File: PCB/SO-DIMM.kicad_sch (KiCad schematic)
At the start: 1 part, among them J1 SODIMM-260_Split

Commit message: Fix broken CM4IO/SODIMM library links and add missing footprints
Both fp-lib-table and sym-lib-table pointed to other collaborators'
absolute local paths (a Windows user path and a Linux path), so the
CM4IO and SODIMM libraries could not resolve on this machine at all.
Repointed both tables at the project's own libraries/ folder using
${KIPRJMOD}-relative paths.

- Added the missing SODIMM_DDR4_EDGE footprint (260-pin card edge)
  and split the combined CM4 mezzanine footprint into
  Raspberry-Pi-4-Compute-Module-A/-B to match the schematic's
  existing per-connector pin numbering (1-100 / 101-200)
- Added Connectors.pretty and MCP25625T_E_ML.pretty footprint
  libraries that were referenced but never committed
- Moved the Mezzanine_A/Mezzanine_B symbols out of the orphaned
  "kai-library" reference (which pointed to no actual file) into
  the existing CM4IO symbol library
- Corrected Module1/Module2 MPN/Digi-Key part numbers to the
  primary DF40HC(3.0)-100DS-0.4V variant, keeping the old
  DF40C-100DS-0.4V values as (Alt) fields
- Reverted an in-progress SO-DIMM.kicad_sch rework that had
  misrouted 8 PCIe signals to the wrong physical pins and silently
  disconnected the CSI/USB3 nets, restoring the known-good pinout
  while keeping the CM4IO footprint rename

Co-Authored-By: Claude Sonnet 5 <noreply@anthropic.com>
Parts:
- J1: footprint kai's library:SODIMM_DDR4_EDGE -> CM4IO:SODIMM_DDR4_EDGE
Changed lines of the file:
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@@
 			)
 		)
-		(property "Footprint" "kai's library:SODIMM_DDR4_EDGE"
+		(property "Footprint" "CM4IO:SODIMM_DDR4_EDGE"
 			(at 396.24 156.21 0)
 			(hide yes)
@@
 			)
 		)
-		(property "Footprint" "kai's library:SODIMM_DDR4_EDGE"
+		(property "Footprint" "CM4IO:SODIMM_DDR4_EDGE"
 			(at 147.32 148.59 0)
 			(hide yes)
@@
 			)
 		)
-		(property "Footprint" "kai's library:SODIMM_DDR4_EDGE"
+		(property "Footprint" "CM4IO:SODIMM_DDR4_EDGE"
 			(at 229.87 71.12 0)
 			(hide yes)
@@
 			)
 		)
-		(property "Footprint" "kai's library:SODIMM_DDR4_EDGE"
+		(property "Footprint" "CM4IO:SODIMM_DDR4_EDGE"
 			(at 312.42 71.12 0)
 			(hide yes)
@@
 			)
 		)
-		(property "Footprint" "kai's library:SODIMM_DDR4_EDGE"
+		(property "Footprint" "CM4IO:SODIMM_DDR4_EDGE"
 			(at 130.81 62.23 0)
 			(hide yes)
@@
 			)
 		)
-		(property "Footprint" "kai's library:SODIMM_DDR4_EDGE"
+		(property "Footprint" "CM4IO:SODIMM_DDR4_EDGE"
 			(at 394.97 71.12 0)
 			(hide yes)
@@
 			)
 		)
-		(property "Footprint" "kai's library:SODIMM_DDR4_EDGE"
+		(property "Footprint" "CM4IO:SODIMM_DDR4_EDGE"
 			(at 276.86 156.21 0)
 			(hide yes)

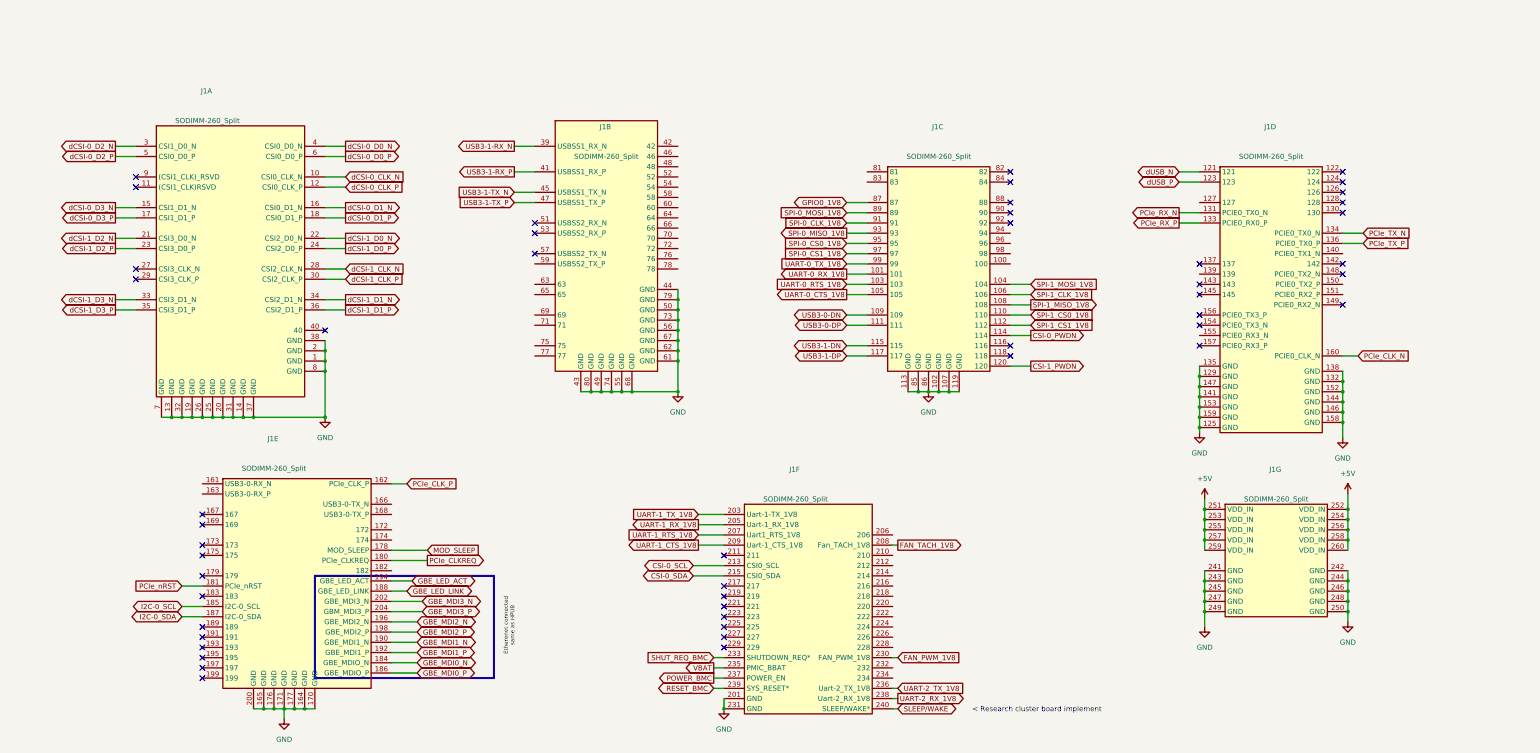
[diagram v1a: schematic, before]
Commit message: Add CAN/PCIe wake signals, drop USB3/CSI-1/most of SPI-1, route GbE pairs
Schematic changes (confirmed intentional):
- Renamed dCSI-0_D2/D3_N/P to CSI-0_D2/D3_N/P (same pins, label cleanup)
- Added CAN_RX/CAN_TX on J1 pins 143/145
- Added PCIe_WAKE_N on J1 pin 179 / Module1 pin 104 (repurposed from
  SPI-1_MOSI_1V8)
- Removed USB3-0 and USB3-1 (both ports entirely), the second CSI
  camera interface (dCSI-1, 10 signals), the remaining 4 SPI-1
  signals, and CSI-0/CSI-1_PWDN

PCB changes:
- Added carrier.kicad_dru with GbE differential pair rules: intra-pair
  skew <=0.25mm (1000BASE-T MDI tolerance) and inter-pair length
  matched to 49.7-50.7mm, both validated against kicad-cli pcb drc
- In-progress length tuning on the 4 GBE_MDI differential pairs

Co-Authored-By: Claude Sonnet 5 <noreply@anthropic.com>
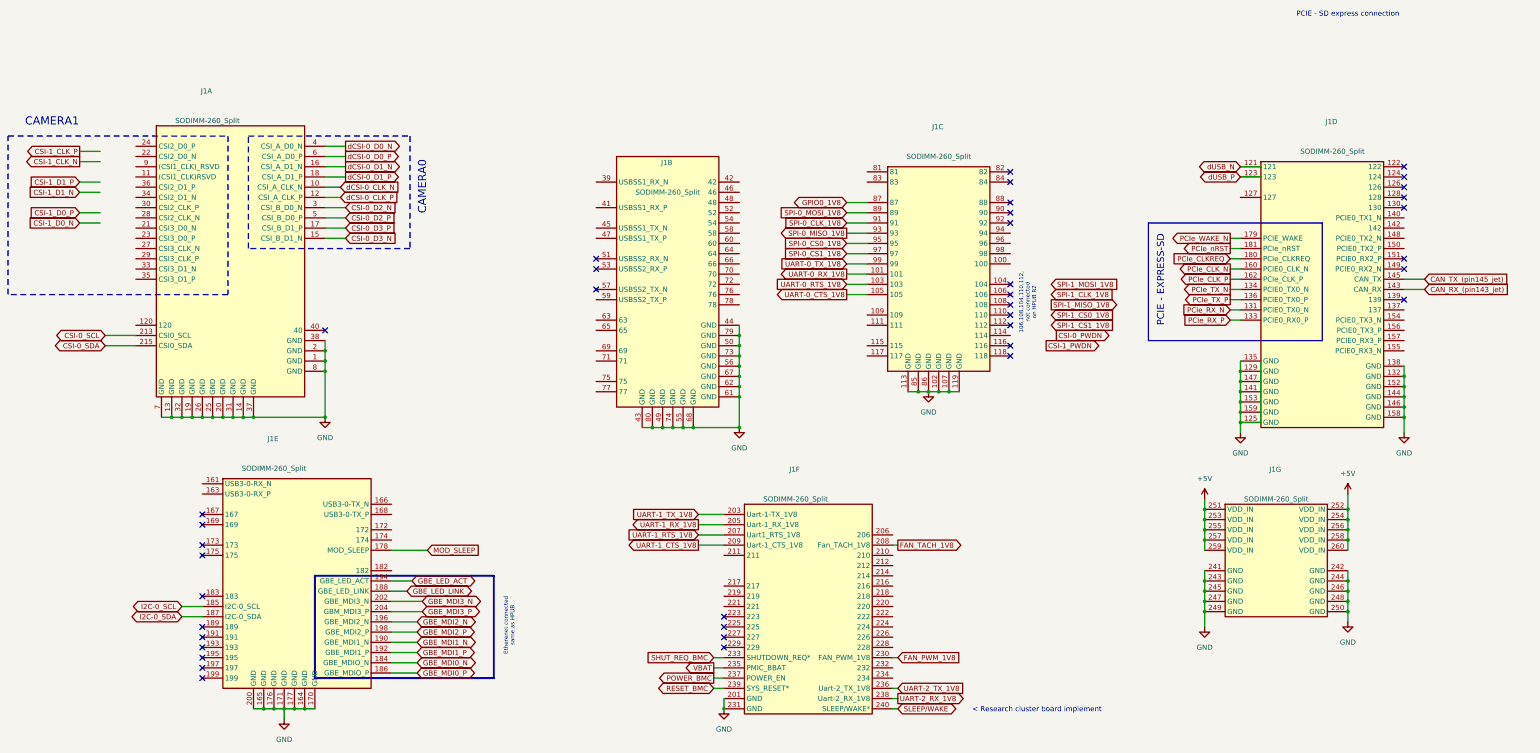
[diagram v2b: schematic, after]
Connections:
- net CSI-0_PWDN: no longer J1.114
- net CSI-0_SCL: now also J1.213 (CSI0_SCL); no longer J1.213 (CSI0_SCL)
- net CSI-0_SDA: now also J1.215 (CSI0_SDA); no longer J1.215 (CSI0_SDA)
- net CSI-1_PWDN: no longer J1.120
- net PCIe_CLKREQ: now also J1.180 (PCIe_CLKREQ); no longer J1.180 (PCIe_CLKREQ)
- net PCIe_CLK_P: now also J1.162 (PCIe_CLK_P); no longer J1.162 (PCIe_CLK_P)
- net PCIe_nRST: now also J1.181 (PCIe_nRST); no longer J1.181 (PCIe_nRST)
- net SPI-1_CLK_1V8: no longer J1.106
- net SPI-1_CS0_1V8: no longer J1.110
- net SPI-1_CS1_1V8: no longer J1.112
- net SPI-1_MISO_1V8: no longer J1.108
- net SPI-1_MOSI_1V8: no longer J1.104
- net CAN_RX_(pin143_jet): now reaches J1.143 (CAN_RX)
- net CAN_TX_(pin145_jet): now reaches J1.145 (CAN_TX)
- net USB3-0-DN: no longer names the net of J1.109
- net USB3-0-DP: no longer names the net of J1.111
- net USB3-1-DN: no longer names the net of J1.115
- net USB3-1-DP: no longer names the net of J1.117
- net USB3-1-RX_N: no longer names the net of J1.39 (USBSS1_RX_N)
- net USB3-1-RX_P: no longer names the net of J1.41 (USBSS1_RX_P)
- net USB3-1-TX_N: no longer names the net of J1.45 (USBSS1_TX_N)
- net USB3-1-TX_P: no longer names the net of J1.47 (USBSS1_TX_P)
- net dCSI-0_D2_N renamed CSI-0_D2_N
- net dCSI-0_D2_P renamed CSI-0_D2_P
- net dCSI-0_D3_N renamed CSI-0_D3_N
- net dCSI-0_D3_P renamed CSI-0_D3_P
- net dCSI-1_CLK_N: no longer names the net of J1.28 (CSI2_CLK_N)
- net dCSI-1_CLK_P: no longer names the net of J1.30 (CSI2_CLK_P)
- net dCSI-1_D0_N: no longer names the net of J1.22 (CSI2_D0_N)
- net dCSI-1_D0_P: no longer names the net of J1.24 (CSI2_D0_P)
- net dCSI-1_D1_N: no longer names the net of J1.34 (CSI2_D1_N)
- net dCSI-1_D1_P: no longer names the net of J1.36 (CSI2_D1_P)
- net dCSI-1_D2_N: no longer names the net of J1.21 (CSI3_D0_N)
- net dCSI-1_D2_P: no longer names the net of J1.23 (CSI3_D0_P)
- net dCSI-1_D3_N: no longer names the net of J1.33 (CSI3_D1_N)
- net dCSI-1_D3_P: no longer names the net of J1.35 (CSI3_D1_P)
- new net PCIe_WAKE_N: J1.179 (PCIE_WAKE)
- no-connect marks 49 -> 39
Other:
- note added: "106,108,104,110,112, not connected on HPUB R2"
- note added: "CAMERA0"
- note added: "CAMERA1"
- note added: "PCIE - EXPRESS-SD"
- note added: "PCIE - SD express connection"
- moved on the sheet: J1B

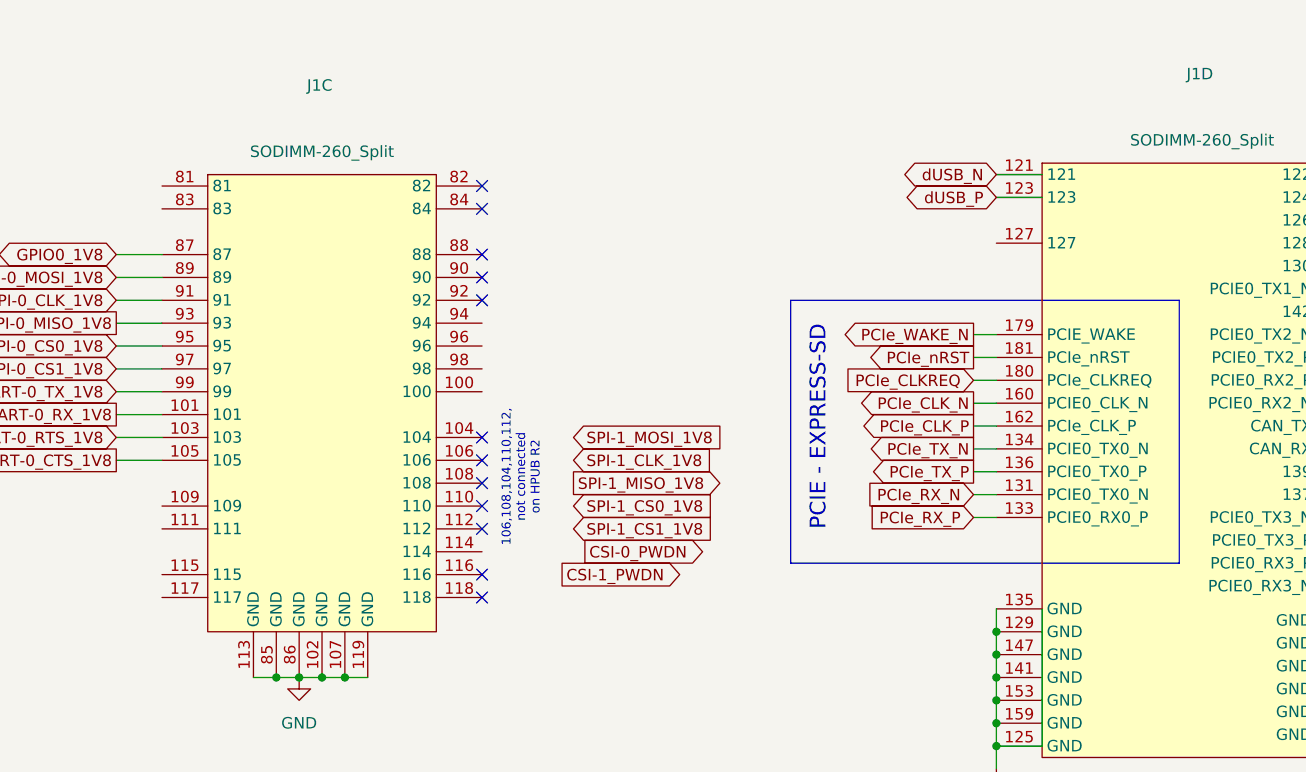
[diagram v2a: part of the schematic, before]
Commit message: Recover crashed sheet hierarchy, add MCP25625 CAN transceiver
KiCad crashed while USB_HUB and CAN PHY sheets were mid-rename, leaving
carrier.kicad_sch pointing at USB.kicad_sch and CAN_PHY.kicad_sch, neither
of which existed on disk. Restored USB_HUB by recovering its content from
the orphaned untitled.kicad_sch (still had the USB2514B/ECS crystal fixes
intact), and created a blank CAN_PHY.kicad_sch so the hierarchy loads
cleanly. The crash also truncated fp-lib-table/sym-lib-table back to an
earlier state; re-added the missing USB2514B/ECS/MCP25625 entries.

Also placed the MCP25625 CAN transceiver, moved its library into
libraries/MCP25625T_E_ML/ to match the convention used by the other custom
parts, and fixed its footprint field to include the library nickname
(it was saved without one, same class of bug as the earlier USB2514B fix).

Co-Authored-By: Claude Sonnet 5 <noreply@anthropic.com>
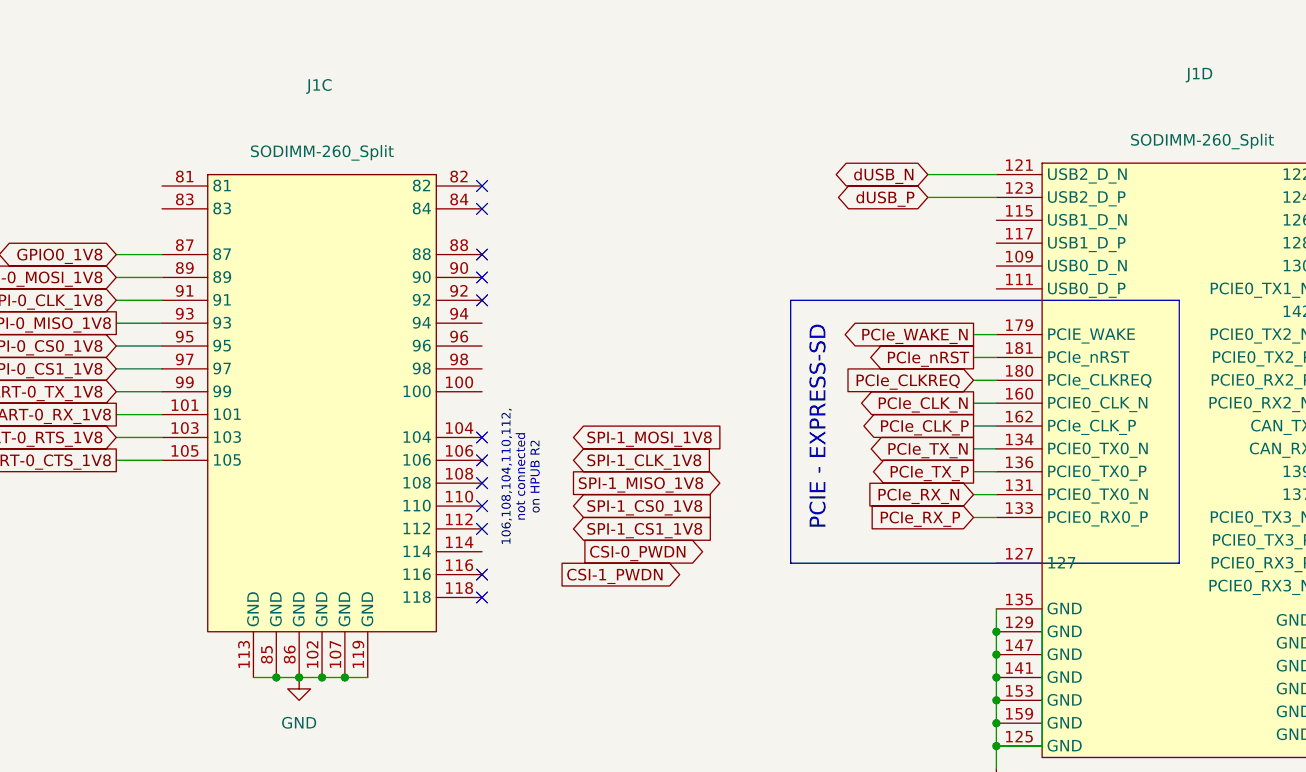
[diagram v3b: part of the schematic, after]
